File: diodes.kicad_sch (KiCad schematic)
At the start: 12 parts

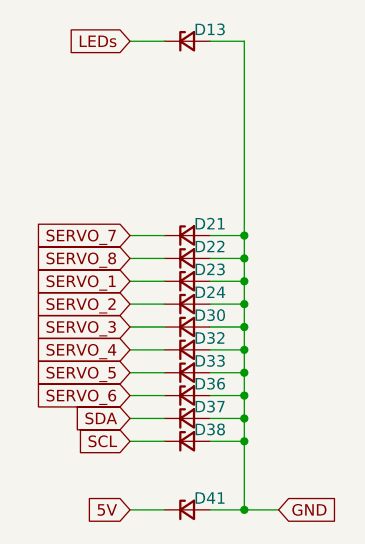
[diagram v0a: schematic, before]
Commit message: update BOM + add big capas (do not take DNP into account)
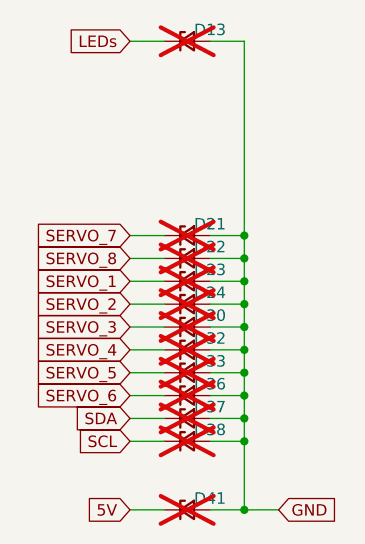
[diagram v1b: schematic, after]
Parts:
- D13, D21, D22, D23, D24, D30, D32, D33, D36, D37, D38, D41: now not fitted
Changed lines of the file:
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@@
 		(in_bom yes)
 		(on_board yes)
-		(dnp no)
+		(dnp yes)
 		(property "Reference" "D21"
 			(at 120.65 95.25 0)
@@
 		(in_bom yes)
 		(on_board yes)
-		(dnp no)
+		(dnp yes)
 		(property "Reference" "D36"
 			(at 120.65 113.03 0)
@@
 		(in_bom yes)
 		(on_board yes)
-		(dnp no)
+		(dnp yes)
 		(property "Reference" "D32"
 			(at 120.65 107.95 0)
@@
 		(in_bom yes)
 		(on_board yes)
-		(dnp no)
+		(dnp yes)
 		(property "Reference" "D38"
 			(at 120.65 118.11 0)
@@
 		(in_bom yes)
 		(on_board yes)
-		(dnp no)
+		(dnp yes)
 		(property "Reference" "D41"
 			(at 120.65 125.73 0)
@@
 		(in_bom yes)
 		(on_board yes)
-		(dnp no)
+		(dnp yes)
 		(property "Reference" "D33"
 			(at 120.65 110.49 0)
@@
 		(in_bom yes)
 		(on_board yes)
-		(dnp no)
+		(dnp yes)
 		(property "Reference" "D30"
 			(at 120.65 105.41 0)
@@
 		(in_bom yes)
 		(on_board yes)
-		(dnp no)
+		(dnp yes)
 		(property "Reference" "D37"
 			(at 120.65 115.57 0)
@@
 		(in_bom yes)
 		(on_board yes)
-		(dnp no)
+		(dnp yes)
 		(property "Reference" "D13"
 			(at 120.65 73.66 0)
@@
 		(in_bom yes)
 		(on_board yes)
-		(dnp no)
+		(dnp yes)
 		(property "Reference" "D23"
 			(at 120.65 100.33 0)
@@
 		(in_bom yes)
 		(on_board yes)
-		(dnp no)
+		(dnp yes)
 		(property "Reference" "D24"
 			(at 120.65 102.87 0)
@@
 		(in_bom yes)
 		(on_board yes)
-		(dnp no)
+		(dnp yes)
 		(property "Reference" "D22"
 			(at 120.65 97.79 0)

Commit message: fix DNP (was just for checking what was to be bought)
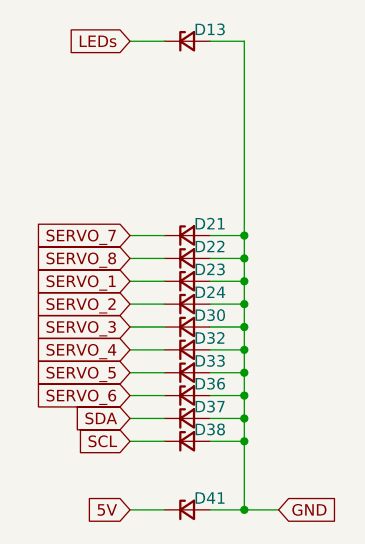
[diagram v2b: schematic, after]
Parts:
- D13, D21, D22, D23, D24, D30, D32, D33, D36, D37, D38, D41: now fitted
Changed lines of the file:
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@@
 		(in_bom yes)
 		(on_board yes)
-		(dnp yes)
+		(dnp no)
 		(property "Reference" "D21"
 			(at 120.65 95.25 0)
@@
 		(in_bom yes)
 		(on_board yes)
-		(dnp yes)
+		(dnp no)
 		(property "Reference" "D36"
 			(at 120.65 113.03 0)
@@
 		(in_bom yes)
 		(on_board yes)
-		(dnp yes)
+		(dnp no)
 		(property "Reference" "D32"
 			(at 120.65 107.95 0)
@@
 		(in_bom yes)
 		(on_board yes)
-		(dnp yes)
+		(dnp no)
 		(property "Reference" "D38"
 			(at 120.65 118.11 0)
@@
 		(in_bom yes)
 		(on_board yes)
-		(dnp yes)
+		(dnp no)
 		(property "Reference" "D41"
 			(at 120.65 125.73 0)
@@
 		(in_bom yes)
 		(on_board yes)
-		(dnp yes)
+		(dnp no)
 		(property "Reference" "D33"
 			(at 120.65 110.49 0)
@@
 		(in_bom yes)
 		(on_board yes)
-		(dnp yes)
+		(dnp no)
 		(property "Reference" "D30"
 			(at 120.65 105.41 0)
@@
 		(in_bom yes)
 		(on_board yes)
-		(dnp yes)
+		(dnp no)
 		(property "Reference" "D37"
 			(at 120.65 115.57 0)
@@
 		(in_bom yes)
 		(on_board yes)
-		(dnp yes)
+		(dnp no)
 		(property "Reference" "D13"
 			(at 120.65 73.66 0)
@@
 		(in_bom yes)
 		(on_board yes)
-		(dnp yes)
+		(dnp no)
 		(property "Reference" "D23"
 			(at 120.65 100.33 0)
@@
 		(in_bom yes)
 		(on_board yes)
-		(dnp yes)
+		(dnp no)
 		(property "Reference" "D24"
 			(at 120.65 102.87 0)
@@
 		(in_bom yes)
 		(on_board yes)
-		(dnp yes)
+		(dnp no)
 		(property "Reference" "D22"
 			(at 120.65 97.79 0)
